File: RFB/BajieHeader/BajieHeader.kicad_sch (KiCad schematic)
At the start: 40 parts, among them J1 Conn_02x25_Odd_Even, J2 Conn_01x16_MountingPin, J3 Conn_02x06_Odd_Even, J4 Conn_01x02_Male, J5 Conn_01x02_Male, J6 Conn_01x04, J7 Conn_01x03_Male, U1 LMR51430, U2 LMR51430, U3 ISO1044UB, U4 LMR51430

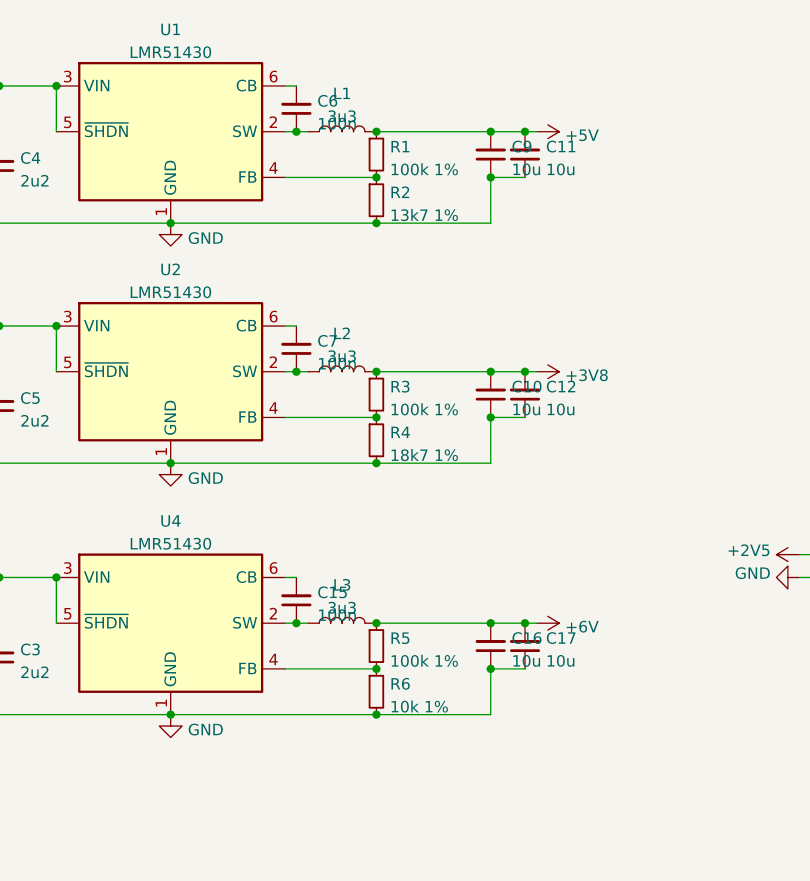
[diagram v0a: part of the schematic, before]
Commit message: w
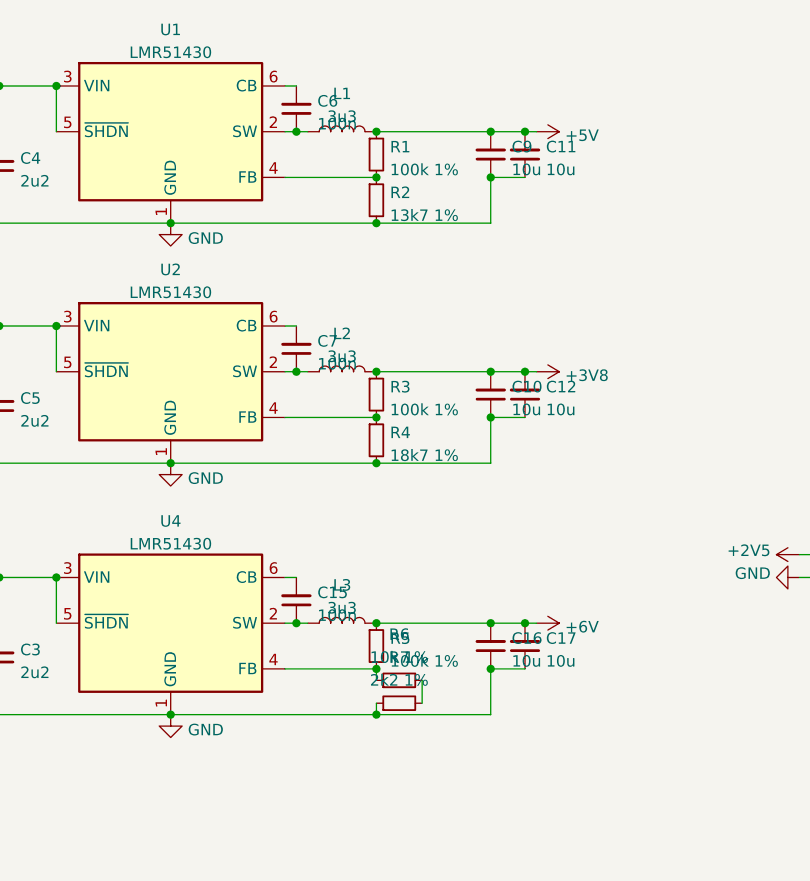
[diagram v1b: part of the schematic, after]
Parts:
- added R7: 2k2 1%, Resistor_SMD:R_0402_1005Metric, symbol Device:R_Small
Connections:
- net GND: now also R7.1; no longer R6.2
- new net: R6.2, R7.2
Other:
- moved on the sheet: R6
